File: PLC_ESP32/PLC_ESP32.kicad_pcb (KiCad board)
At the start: 2 copper layers, 100 x 100 mm, 128 parts, among them J1 USB_B_Micro, J10 Salidas Analogicas, J11 Salida PWM, J12 UART_SERIE, J13 Entrada Digital, J14 Entrada Digital, J15 Entrada Digital, J16 Entrada Analogica, J2 Terminales Reles, J3 Terminales Reles, J4 Terminales Triacs, J5 Terminales Triacs, J6 Entrada_24VDC, J7 PANTALLA LCD I2C, J8 DS3231, J9 PANTALLA OLED, K1 SANYOU_SRD_Form_C, K2 SANYOU_SRD_Form_C, K3 SANYOU_SRD_Form_C, Q1 SS8050-G, Q10 BT136-500, Q2 SS8050-G, Q3 2N2222A, Q4 2N2222A, Q5 2N2222A, Q6 BT136-500, Q7 BT136-500, Q8 BT136-500, Q9 BT136-500, SW1 SW_Push, SW2 SW_Push, U1 AMS1117-3.3, U10 MOC3021M, U11 MOC3021M, U12 LM7805_TO220, U13 LM7810_TO220, U14 PC817, U15 LM358, U16 PC817, U17 PC817, U18 PC817, U2 CP2102N-A01-GQFN28, U3 ESP32-WROOM-32, U4 PC817, U5 PC817, U6 PC817, U7 MOC3021M, U8 MOC3021M, U9 MOC3021M

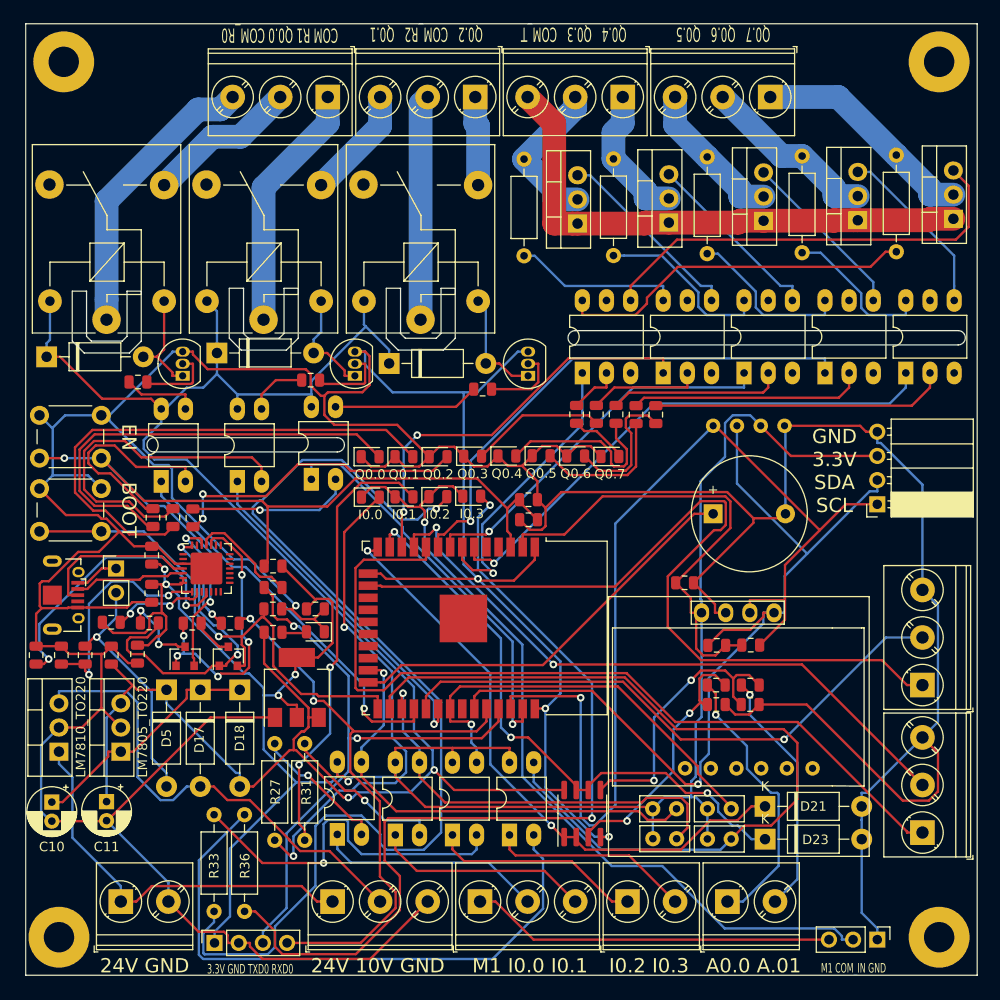
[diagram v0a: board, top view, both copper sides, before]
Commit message: -
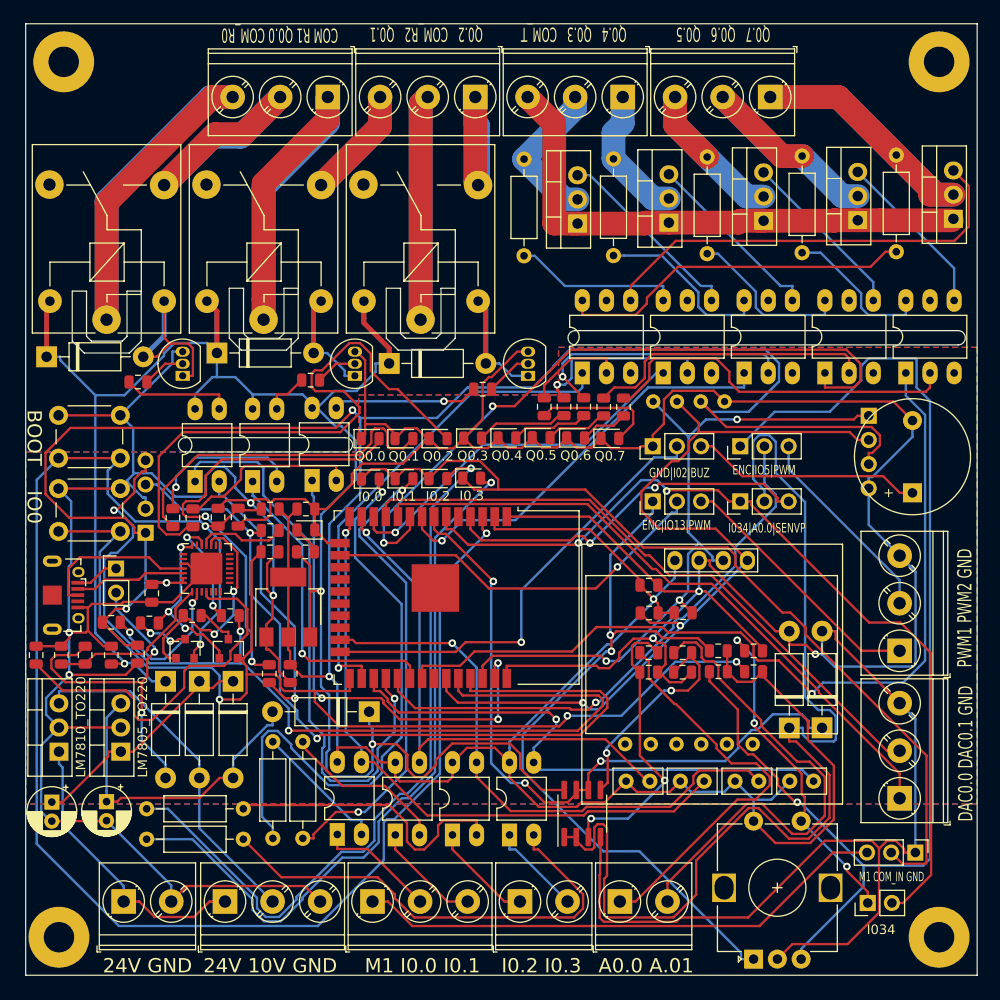
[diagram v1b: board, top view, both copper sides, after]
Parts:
- added D25: BAT760-7 30V 1A, Diode_THT:D_DO-41_SOD81_P10.16mm_Horizontal, F.Cu at (116.1, 137.3)
- added JP3: IO2, Connector_PinHeader_2.54mm:PinHeader_1x03_P2.54mm_Vertical, F.Cu at (145.9, 109.4)
- added JP4: IO13, Connector_PinHeader_2.54mm:PinHeader_1x03_P2.54mm_Vertical, F.Cu at (145.9, 115.2)
- added JP5: IO5, Connector_PinHeader_2.54mm:PinHeader_1x03_P2.54mm_Vertical, F.Cu at (155.1, 109.4)
- added JP6: IO13, Connector_PinHeader_2.54mm:PinHeader_1x03_P2.54mm_Vertical, F.Cu at (155.1, 115.2)
- added JP7: IO34, Connector_PinHeader_2.54mm:PinHeader_1x02_P2.54mm_Vertical, F.Cu at (168.5, 157.4)
- added R29: 10K(5%), Resistor_SMD:R_0805_2012Metric, F.Cu at (152.8, 130.9)
- added R34: 10K(5%), Resistor_SMD:R_0805_2012Metric, F.Cu at (152.8, 133.1)
- added R39: 10K(5%), Resistor_SMD:R_0805_2012Metric, F.Cu at (156.5, 130.9)
- added R40: 10K(5%), Resistor_SMD:R_0805_2012Metric, F.Cu at (156.5, 133.1)
- added REF5: KiCad-Logo2_20mm_SilkScreen, Symbol:KiCad-Logo2_20mm_SilkScreen, B.Cu at (112.3, 127.2)
- added SW3: Rotary_Encoder_Switch, Rotary_Encoder:RotaryEncoder_Alps_EC12E-Switch_Vertical_H20mm, F.Cu at (156.5, 163.3)
- J12: footprint Connector_PinSocket_2.54mm:PinSocket_1x04_P2.54mm_Vertical -> Connector_PinSocket_2.54mm:PinSocket_1x04_P2.54mm_Horizontal; moved to B.Cu
- J7: moved to B.Cu
- moved J12 43.7 mm to (92.6, 118.5), turned to 0 degrees
- moved C5 32.7 mm to (100.2, 116.9), turned to 90 degrees
- moved C9 30.5 mm to (102.3, 116.8), turned to 270 degrees
- moved BZ1 21.1 mm to (173.2, 114.3), turned to 90 degrees
- moved R11 20.5 mm to (105.6, 133.3), turned to 90 degrees
- moved C3 19.1 mm to (107.8, 133.3), turned to 90 degrees
- moved D23 13.1 mm to (163.7, 139.0), turned to 90 degrees
- moved J15 11.3 mm to (131.9, 157.2)
- moved J16 11.3 mm to (142.4, 157.2)
- moved J13 11.3 mm to (101.0, 157.2)
- moved J14 11.3 mm to (116.5, 157.2)
- moved D1 10.7 mm to (109.5, 118.2)
- moved C15 10.6 mm to (160.3, 144.6)
- moved C6 10.5 mm to (109.5, 116.0)
- moved JP2 9.99 mm to (173.5, 152.1)
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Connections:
- BZ1 pad 1: /Control/IO2 -> Net-(BZ1-Pad1)
- C11 pad 1: +5V -> Net-(C11-Pad1)
- D18 pad 2: +5V -> Net-(C11-Pad1)
- J11 pad 1: /Control/IO13 -> /Control/IO13_PWM
- J11 pad 2: /Control/IO5 -> /Control/IO5_PWM
- U12 pad 3: +5V -> Net-(C11-Pad1)
- U3 pad 13: /Control/A0.1 -> /Control/I0.1
- U3 pad 14: /Control/A0.0 -> /Control/I0.0
- U3 pad 23: /Control/I0.0 -> /Control/I0.2
- U3 pad 26: /Control/I0.3 -> /Control/Q0.7
- U3 pad 27: /Control/I0.1 -> /Control/I0.3
- U3 pad 31: /Control/I0.2 -> /Control/Q0.6
- U3 pad 6: /Control/Q0.6 -> /Control/IO34
- U3 pad 7: /Control/Q0.7 -> /Control/A0.1
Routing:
- net /Control/B_ENCODER: track 0.00 -> 123.9 mm, vias 0 -> 1
- net /Control/IO34: track 0.00 -> 92.3 mm, vias 0 -> 2
- net +3V3: track 282.8 -> 372.5 mm
- net /Control/A_ENCODER: track 0.00 -> 78.7 mm, vias 0 -> 2
- net /Control/EN: track 97.4 -> 170.5 mm, vias 2 -> 3
- net /Control/IO0: track 54.8 -> 118.0 mm, vias 1 -> 3
- net /Control/A0.0: track 63.7 -> 111.9 mm, vias 2 -> 0
- net /Control/IO13: track 86.7 -> 41.3 mm, vias 0 -> 1
- net /Control/SENSOR_VP: track 0.00 -> 39.3 mm, vias 0 -> 2
- net /Control/SCL: track 112.9 -> 74.3 mm, vias 1 -> 3
- net /Control/Q0.6: track 56.0 -> 92.0 mm
- net /Control/RXD0: track 67.7 -> 103.3 mm, vias 2 -> 3
- net Net-(JP7-Pad1): track 0.00 -> 35.1 mm, vias 0 -> 3
- net Net-(C11-Pad1): track 0.00 -> 34.3 mm
- net Net-(D22-Pad2): track 112.2 -> 79.6 mm
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- added copper zone on B.Cu, net GND
- added copper zone on F.Cu, net GND
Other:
- outline, holes or cut-outs redrawn
- net class Alimentacion added: clearance 0.2, trace_width 0.5, via_dia 0.8, via_drill 0.4
- rule trace_min: 0.2 -> 0.25
- board text added: "DAC0.0 DAC0.1 GND"
- board text added: "ENC|IO13|PWM"
- board text added: "ENC|IO5|PWM"
- board text added: "GND|I02|BUZ"
- board text added: "I034"
- board text added: "I034|A0.0|SENVP"
- board text added: "IO0"
- board text added: "PLC ESP32 V1.0 Agustin Zuliani"
- board text added: "PWM1 PWM2 GND"
- board text removed: "EN"
